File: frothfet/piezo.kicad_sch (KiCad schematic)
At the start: 3 parts, among them Q19 AO3400A

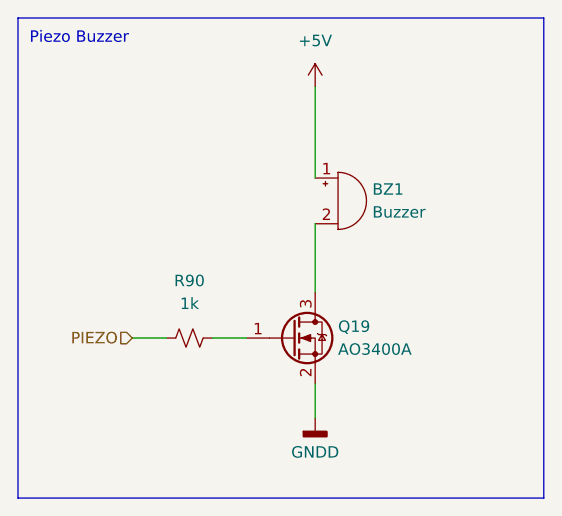
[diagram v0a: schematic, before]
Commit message: piezo resistor
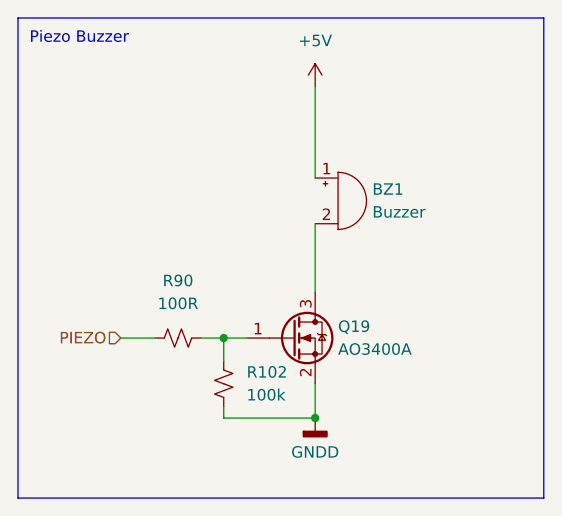
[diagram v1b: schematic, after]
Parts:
- added R102: 100k, Resistor_SMD:R_0603_1608Metric, symbol Device:R_Small_US
- R90: value 1k -> 100R
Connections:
- net GNDD: now also R102.2
- net at Q19.1 (G), R90.1: now also R102.1
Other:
- moved on the sheet: R90
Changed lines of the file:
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@@
 		)
+	)
+	(junction
+		(at 134.62 109.22)
+		(diameter 0)
+		(color 0 0 0 0)
+	)
+	(junction
+		(at 124.46 100.33)
+		(diameter 0)
+		(color 0 0 0 0)
 	)
 	(wire
@@
 	(wire
 		(pts
-			(xy 123.19 100.33) (xy 127 100.33)
-		)
-		(stroke
-			(width 0)
-			(type default)
-		)
-	)
-	(wire
-		(pts
-			(xy 114.3 100.33) (xy 118.11 100.33)
+			(xy 134.62 109.22) (xy 124.46 109.22)
+		)
+		(stroke
+			(width 0)
+			(type default)
+		)
+	)
+	(wire
+		(pts
+			(xy 121.92 100.33) (xy 124.46 100.33)
+		)
+		(stroke
+			(width 0)
+			(type default)
+		)
+	)
+	(wire
+		(pts
+			(xy 124.46 109.22) (xy 124.46 107.95)
+		)
+		(stroke
+			(width 0)
+			(type default)
+		)
+	)
+	(wire
+		(pts
+			(xy 113.03 100.33) (xy 116.84 100.33)
+		)
+		(stroke
+			(width 0)
+			(type default)
+		)
+	)
+	(wire
+		(pts
+			(xy 124.46 100.33) (xy 127 100.33)
 		)
 		(stroke
@@
 		(pts
 			(xy 134.62 72.39) (xy 134.62 82.55)
+		)
+		(stroke
+			(width 0)
+			(type default)
+		)
+	)
+	(wire
+		(pts
+			(xy 124.46 100.33) (xy 124.46 102.87)
 		)
 		(stroke
@@
 	(hierarchical_label "PIEZO"
 		(shape input)
-		(at 114.3 100.33 180)
+		(at 113.03 100.33 180)
 		(effects
 			(font
@@
 	(symbol
 		(lib_id "Device:R_Small_US")
-		(at 120.65 100.33 270)
+		(at 124.46 105.41 0)
+		(unit 1)
+		(exclude_from_sim no)
+		(in_bom yes)
+		(on_board yes)
+		(dnp no)
+		(fields_autoplaced yes)
+		(property "Reference" "R102"
+			(at 127 104.1399 0)
+			(effects
+				(font
+					(size 1.27 1.27)
+				)
+				(justify left)
+			)
+		)
+		(property "Value" "100k"
+			(at 127 106.6799 0)
+			(effects
+				(font
+					(size 1.27 1.27)
+				)
+				(justify left)
+			)
+		)
+		(property "Footprint" "Resistor_SMD:R_0603_1608Metric"
+			(at 124.46 105.41 0)
+			(effects
+				(font
+					(size 1.27 1.27)
+				)
+				(hide yes)
+			)
+		)
+		(property "Datasheet" "~"
+			(at 124.46 105.41 0)
+			(effects
+				(font
+					(size 1.27 1.27)
+				)
+				(hide yes)
+			)
+		)
+		(property "Description" ""
+			(at 124.46 105.41 0)
+			(effects
+				(font
+					(size 1.27 1.27)
+				)
+				(hide yes)
+			)
+		)
+		(pin "1"
+		)
+		(pin "2"
+		)
+		(instances
+			(project "frothfet"
+				(path "/c83c6236-96e9-46ad-9d7a-9e2efa4a7966/13bd1484-e1d0-414c-b70b-256f3904dbbc"
+					(reference "R102")
+					(unit 1)
+				)
+			)
+		)
+	)
+	(symbol
+		(lib_id "Device:R_Small_US")
+		(at 119.38 100.33 270)
 		(unit 1)
 		(exclude_from_sim no)
@@
 		(fields_autoplaced yes)
 		(property "Reference" "R90"
-			(at 120.65 93.98 90)
-			(effects
-				(font
-					(size 1.27 1.27)
-				)
-			)
-		)
-		(property "Value" "1k"
-			(at 120.65 96.52 90)
+			(at 119.38 93.98 90)
+			(effects
+				(font
+					(size 1.27 1.27)
+				)
+			)
+		)
+		(property "Value" "100R"
+			(at 119.38 96.52 90)
 			(effects
 				(font
@@
 		)
 		(property "Footprint" "Resistor_SMD:R_0603_1608Metric"
-			(at 120.65 100.33 0)
+			(at 119.38 100.33 0)
 			(effects
 				(font
@@
 		)
 		(property "Datasheet" "~"
-			(at 120.65 100.33 0)
+			(at 119.38 100.33 0)
 			(effects
 				(font
@@
 		)
 		(property "Description" ""
-			(at 120.65 100.33 0)
-			(effects
-				(font
-					(size 1.27 1.27)
-				)
-				(hide yes)
-			)
-		)
-		(property "LCSC" ""
-			(at 120.65 100.33 0)
-			(effects
-				(font
-					(size 1.27 1.27)
-				)
-				(hide yes)
-			)
-		)
-		(property "ALT" ""
-			(at 120.65 100.33 0)
-			(effects
-				(font
+			(at 119.38 100.33 0)
+			(effects
+				(font
